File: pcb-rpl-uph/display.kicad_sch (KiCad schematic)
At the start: 1 part, among them J15 20879-040E-01

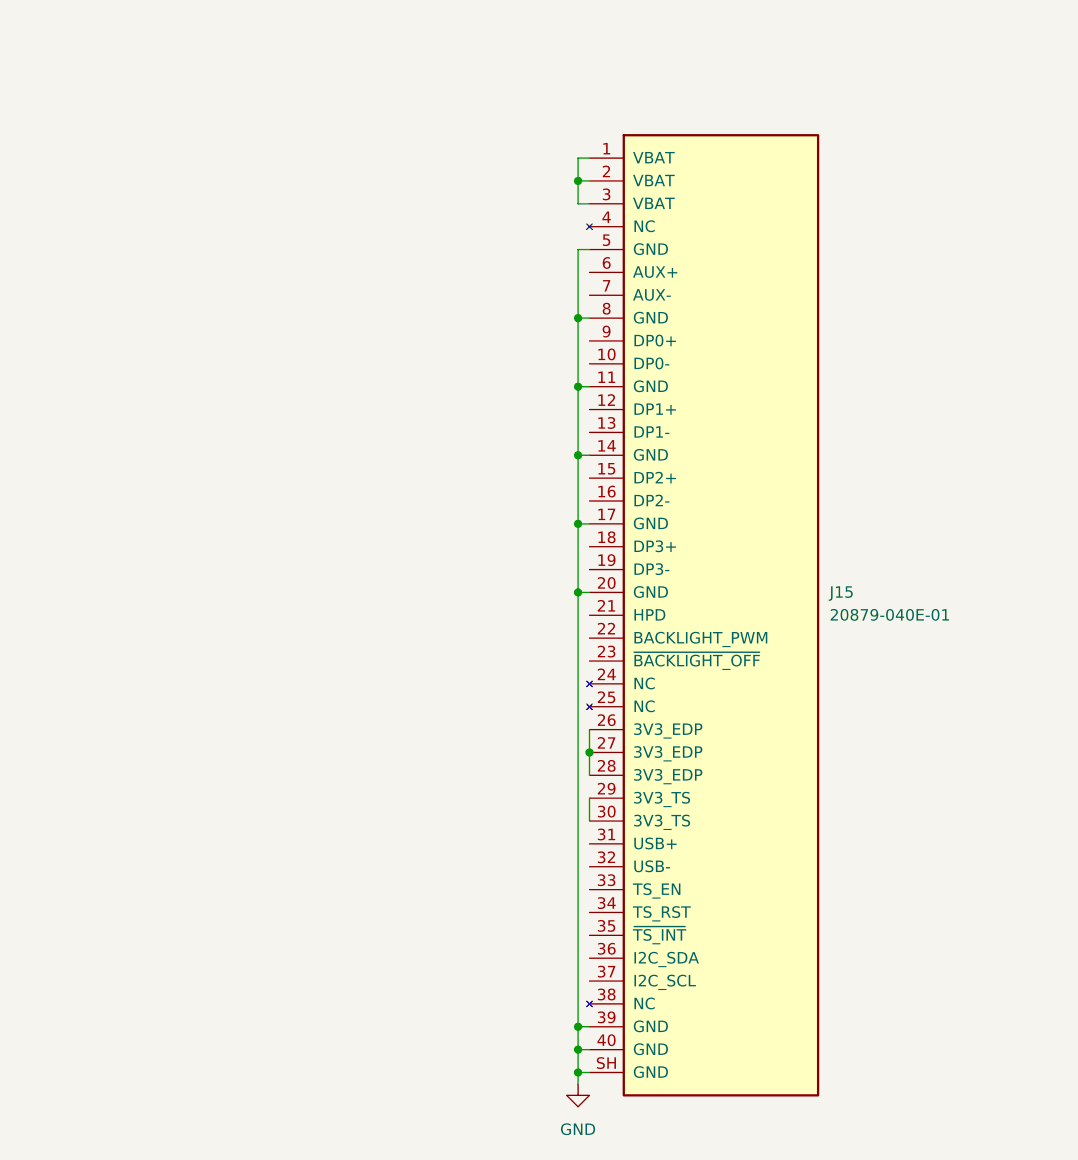
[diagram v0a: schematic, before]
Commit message: add display connector
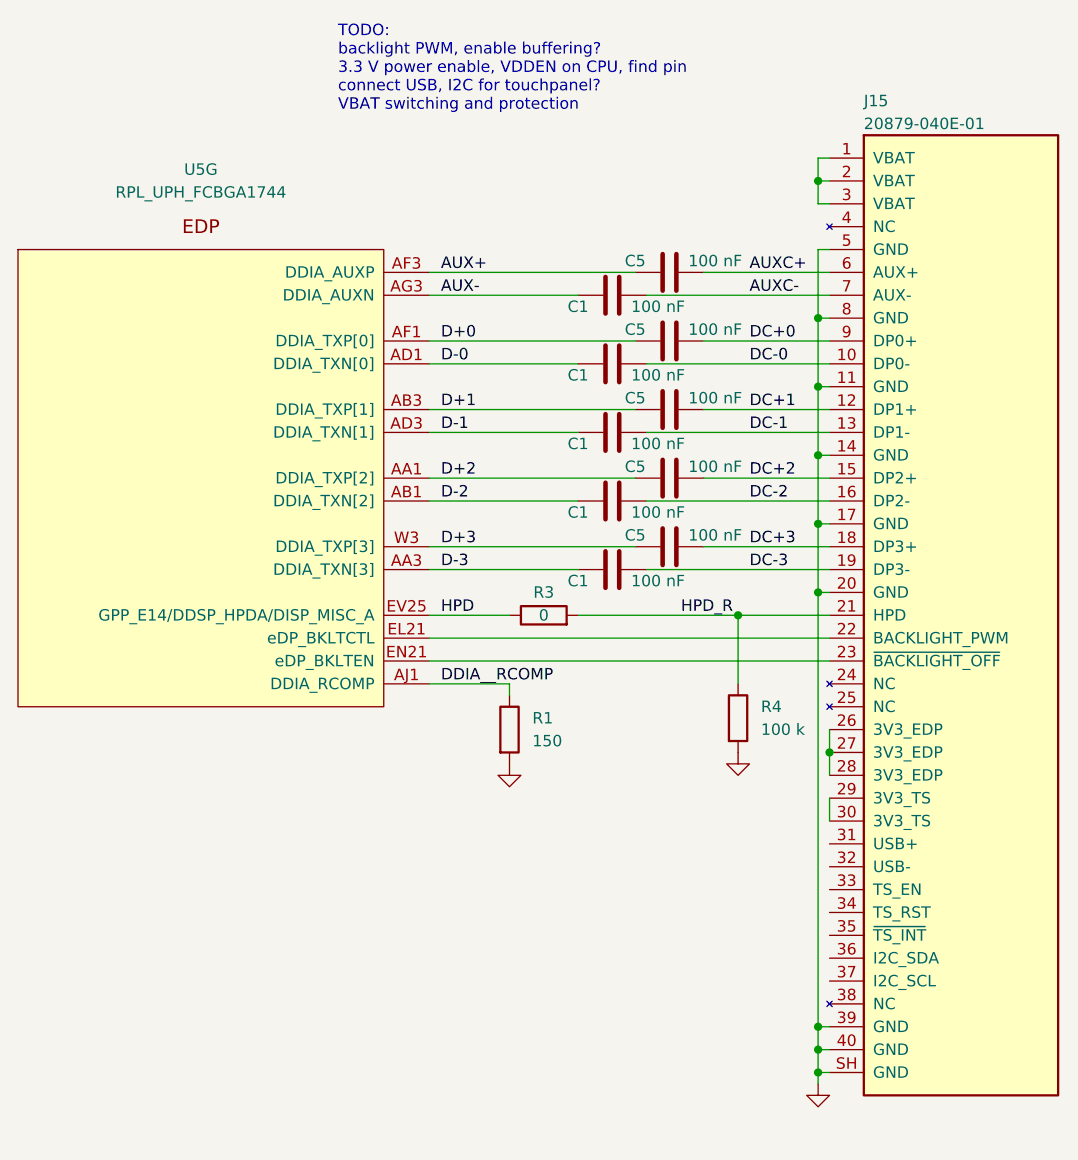
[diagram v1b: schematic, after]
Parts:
- added C1 (x5), C5 (x5): 100 nF, local:C_0201_0603Metric, symbol Device:C
- added R1: 150, local:R_0201_0603Metric, symbol Device:R
- added R3: 0, local:R_0201_0603Metric, symbol Device:R
- added R4: 100 k, local:R_0201_0603Metric, symbol Device:R
- added U5: RPL_UPH_FCBGA1744, local:RPL_UPH_FCBGA1744, symbol local:RPL_UPH_FCBGA1744
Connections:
- net GND: now also R1.2, R4.2
- net DC-0: now reaches J15.10 (DP0-)
- net DC-0: now also C1.2
- net DC+1: now reaches J15.12 (DP1+)
- net DC+1: now also C5.2
- net DC-1: now reaches J15.13 (DP1-)
- net DC-1: now also C1.2
- net DC+2: now reaches J15.15 (DP2+)
- net DC+2: now also C5.2
- net DC-2: now reaches J15.16 (DP2-)
- net DC-2: now also C1.2
- net DC+3: now reaches J15.18 (DP3+)
- net DC+3: now also C5.2
- net DC-3: now reaches J15.19 (DP3-)
- net DC-3: now also C1.2
- net HPD_R: now reaches J15.21 (HPD)
- net HPD_R: now also R3.2, R4.1
- net at J15.22 (BACKLIGHT_PWM): now also U5.EL21 (eDP_BKLTCTL)
- net at J15.23 (~{BACKLIGHT_OFF}): now also U5.EN21 (eDP_BKLTEN)
- net AUXC+: now reaches J15.6 (AUX+)
- net AUXC+: now also C5.2
- net AUXC-: now reaches J15.7 (AUX-)
- net AUXC-: now also C1.2
- net DC+0: now reaches J15.9 (DP0+)
- net DC+0: now also C5.2
- new net AUX+: C5.1, U5.AF3 (DDIA_AUXP)
- new net AUX-: C1.1, U5.AG3 (DDIA_AUXN)
- new net D+0: C5.1, U5.AF1 (DDIA_TXP[0])
- new net D+1: C5.1, U5.AB3 (DDIA_TXP[1])
- new net D+2: C5.1, U5.AA1 (DDIA_TXP[2])
- new net D+3: C5.1, U5.W3 (DDIA_TXP[3])
- new net D-0: C1.1, U5.AD1 (DDIA_TXN[0])
- new net D-1: C1.1, U5.AD3 (DDIA_TXN[1])
- new net D-2: C1.1, U5.AB1 (DDIA_TXN[2])
- new net D-3: C1.1, U5.AA3 (DDIA_TXN[3])
- new net DDIA__RCOMP: R1.1, U5.AJ1 (DDIA_RCOMP)
- new net HPD: R3.1, U5.EV25 (GPP_E14/DDSP_HPDA/DISP_MISC_A)
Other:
- note added: "TODO: backlight PWM, enable buffering? 3.3 V power enable, VDDEN on CPU, find pin connect USB, I2C for touchpanel? VBAT switching and protection"
- moved on the sheet: J15
